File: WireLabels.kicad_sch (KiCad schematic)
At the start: 0 parts

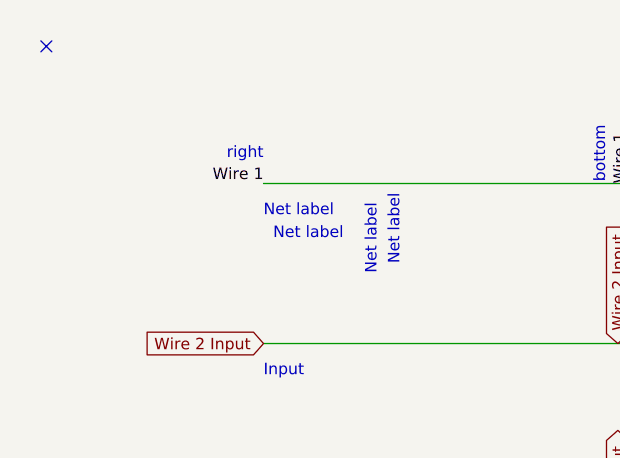
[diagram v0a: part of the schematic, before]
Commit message: blah
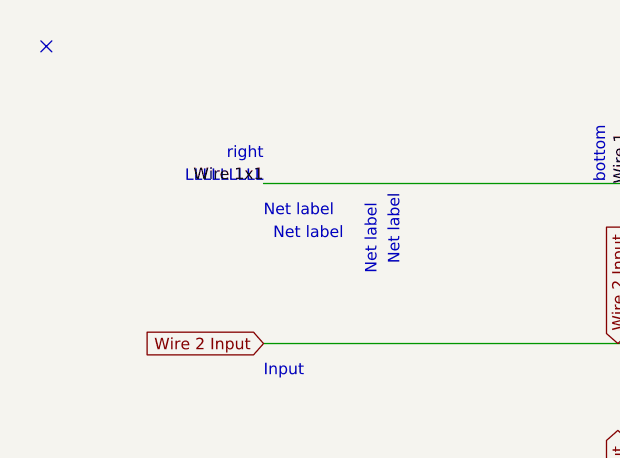
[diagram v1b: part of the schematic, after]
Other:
- note added: "LLLLLLLLL"
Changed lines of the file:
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@@
     (effects (font (size 1.27 1.27)) (justify left bottom))
+  )
+  (text "LLLLLLLLL" (at 90.17 52.07 180)
+    (effects (font (size 1.27 1.27)) (justify right bottom))
   )
   (text "Net label" (at 99.06 58.42 180)
@@
     (effects (font (size 1.27 1.27)) (justify left bottom))
   )
-  (label "Wire 1" (at 90.17 52.07 180)
+  (label "Wire 1x1" (at 90.17 52.07 180)
     (effects (font (size 1.27 1.27)) (justify right bottom))
   )
